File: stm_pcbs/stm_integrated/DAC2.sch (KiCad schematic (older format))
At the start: 21 parts, among them P1 BNC, U1 AD8676, U2 AD5791, U3 AD8675

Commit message: working on Kicad of 3rd Dec
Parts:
- C1, C11, C12, C15, C16, C3, C5, C7, C8: symbol C -> device:C
- C10, C13, C14, C2, C4, C6, C9: symbol CP2 -> device:CP1
- P1: symbol BNC -> device:BNC
- R1: symbol R -> device:R
- U1: symbol AD8676 -> ad5791:AD8676
- U2: symbol AD5791 -> ad5791:AD5791
- U3: symbol AD8675 -> ad5791:AD8675
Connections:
- wire segments 111 -> 126
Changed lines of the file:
@@
-EESchema Schematic File Version 2
-LIBS:power
-LIBS:device
-LIBS:transistors
-LIBS:conn
-LIBS:linear
-LIBS:regul
-LIBS:74xx
-LIBS:cmos4000
-LIBS:adc-dac
-LIBS:memory
-LIBS:xilinx
-LIBS:special
-LIBS:microcontrollers
-LIBS:dsp
-LIBS:microchip
-LIBS:analog_switches
-LIBS:motorola
-LIBS:texas
-LIBS:intel
-LIBS:audio
-LIBS:interface
-LIBS:digital-audio
-LIBS:philips
-LIBS:display
-LIBS:cypress
-LIBS:siliconi
-LIBS:opto
-LIBS:atmel
-LIBS:contrib
-LIBS:valves
-LIBS:ad5791
+EESchema Schematic File Version 4
 LIBS:stmshieldfull-cache
-LIBS:powerbrd-cache
-LIBS:LTC1859-cache
-EELAYER 25 0
+EELAYER 26 0
 EELAYER END
 $Descr A4 11693 8268
@@
 $EndDescr
 $Comp
-L AD5791 U2
+L ad5791:AD5791 U2
 U 1 1 5A25EB42
 P 5050 3750
@@
 $EndComp
 $Comp
-L AD8675 U3
+L ad5791:AD8675 U3
 U 1 1 5A25EB49
 P 6750 3400
@@
 $EndComp
 $Comp
-L AD8676 U1
+L ad5791:AD8676 U1
 U 1 1 5A25EB50
 P 4950 1700
@@
 $EndComp
 $Comp
-L AD8676 U1
+L ad5791:AD8676 U1
 U 2 1 5A25EB57
 P 5000 5450
@@
 $EndComp
 $Comp
-L AD8676 U1
+L ad5791:AD8676 U1
 U 3 1 5A25EB5E
 P 7700 5550
@@
 $EndComp
 $Comp
-L BNC P1
+L device:BNC P1
 U 1 1 5A25EB65
 P 7850 3400
@@
 -14V
 $Comp
-L AGND #PWR01
+L power:AGND #PWR01
 U 1 1 5A25EB72
 P 7850 3750
@@
 3.3V
 $Comp
-L AGND #PWR02
+L power:AGND #PWR02
 U 1 1 5A25EB7B
 P 4850 4850
@@
 $EndComp
 $Comp
-L DGND #PWR03
+L power:DGND #PWR03
 U 1 1 5A25EB81
 P 4600 4850
@@
 $EndComp
 $Comp
-L C C3
+L device:C C3
 U 1 1 5A25EB87
 P 5850 2150
@@
 $EndComp
 $Comp
-L AGND #PWR04
+L power:AGND #PWR04
 U 1 1 5A25EB8E
 P 6300 2300
@@
 $EndComp
 $Comp
-L C C5
+L device:C C5
 U 1 1 5A25EB94
 P 6000 4550
@@
 $EndComp
 $Comp
-L AGND #PWR05
+L power:AGND #PWR05
 U 1 1 5A25EB9B
 P 6400 4700
@@
 $EndComp
 $Comp
-L C C1
+L device:C C1
 U 1 1 5A25EBAF
 P 3850 1850
@@
 $EndComp
 $Comp
-L DGND #PWR06
+L power:DGND #PWR06
 U 1 1 5A25EBB6
 P 3600 1650
@@
 $EndComp
 $Comp
-L C C8
+L device:C C8
 U 1 1 5A25EBBC
 P 7350 5550
@@
 $EndComp
 $Comp
-L C C15
+L device:C C15
 U 1 1 5A25EBC3
 P 8750 5400
@@
 $EndComp
 $Comp
-L C C16
+L device:C C16
 U 1 1 5A25EBCA
 P 8750 5950
@@
 $EndComp
 $Comp
-L AGND #PWR07
+L power:AGND #PWR07
 U 1 1 5A25EBD1
 P 9000 5650
@@
 $EndComp
 $Comp
-L AGND #PWR08
+L power:AGND #PWR08
 U 1 1 5A25EBD7
 P 9000 6200
@@
 $EndComp
 $Comp
-L C C7
+L device:C C7
 U 1 1 5A25EBDD
 P 7100 5550
@@
 $EndComp
 $Comp
-L CP2 C13
+L device:CP1 C13
 U 1 1 5A25EBE4
 P 8500 5400
@@
 $EndComp
 $Comp
-L CP2 C14
+L device:CP1 C14
 U 1 1 5A25EBEB
 P 8500 5950
@@
 $EndComp
 $Comp
-L CP2 C6
+L device:CP1 C6
 U 1 1 5A25EBF2
 P 6000 4800
@@
 $EndComp
 $Comp
-L CP2 C4
+L device:CP1 C4
 U 1 1 5A25EBF9
 P 5850 2400
@@
 $EndComp
 $Comp
-L CP2 C2
+L device:CP1 C2
 U 1 1 5A25EC00
 P 4100 1850
@@
 RESET2
 $Comp
-L CP2 C9
+L device:CP1 C9
 U 1 1 5A25EC0E
 P 7400 3050
@@
 $EndComp
 $Comp
-L CP2 C10
+L device:CP1 C10
 U 1 1 5A25EC15
 P 7400 3800
@@
 $EndComp
 $Comp
-L C C11
+L device:C C11
 U 1 1 5A25EC1C
 P 7600 3050
@@
 $EndComp
 $Comp
-L C C12
+L device:C C12
 U 1 1 5A25EC23
 P 7600 3800
@@
 $EndComp
 $Comp
-L AGND #PWR09
+L power:AGND #PWR09
 U 1 1 5A25EC2A
 P 7300 3250
@@
 $EndComp
 $Comp
-L AGND #PWR010
+L power:AGND #PWR010
 U 1 1 5A25EC30
 P 7400 4100
@@
 	5900 3300 6450 3300
 Wire Wire Line
-	7050 3400 7700 3400
+	7050 3400 7150 3400
 Wire Wire Line
 	4900 1300 4900 1450
@@
 	4900 5700 4900 5850
 Wire Wire Line
-	7250 5200 7800 5200
-Wire Wire Line
-	7250 5900 7800 5900
+	7250 5200 7600 5200
 Wire Wire Line
 	6450 3500 5900 3500
@@
 Connection ~ 7150 3400
 Wire Wire Line
-	6750 3050 6950 3050
-Wire Wire Line
-	6750 3750 6900 3750
+	6750 3050 6850 3050
+Wire Wire Line
+	6750 3750 6850 3750
 Wire Wire Line
 	7850 3600 7850 3750
 Wire Wire Line
-	5600 2000 5600 2300
+	5600 2000 5600 2150
 Wire Wire Line
 	5300 4650 5300 4800
@@
 	4800 2350 4800 2550
 Wire Wire Line
-	4200 2350 4800 2350
+	4200 2350 4450 2350
 Wire Wire Line
 	4650 2350 4650 2550
@@
 Connection ~ 5600 2250
 Wire Wire Line
-	6050 2150 6050 2400
+	6050 2150 6050 2250
 Wire Wire Line
 	6050 2250 6300 2250
@@
 	5300 4650 5800 4650
 Wire Wire Line
-	5800 4550 5800 4800
-Wire Wire Line
-	6200 4550 6200 4800
+	5800 4550 5800 4650
+Wire Wire Line
+	6200 4550 6200 4650
 Connection ~ 5800 4650
 Wire Wire Line
@@
 Connection ~ 6200 4650
 Wire Wire Line
-	3850 1650 4100 1650
-Wire Wire Line
-	3850 2050 4100 2050
-Wire Wire Line
-	3950 2050 4450 2050
+	3850 1650 3950 1650
 Wire Wire Line
 	4450 2050 4450 2350
 Connection ~ 4450 2350
-Connection ~ 3950 2050
 Wire Wire Line
 	3950 1650 3950 1400
@@
 Connection ~ 3950 1650
 Wire Wire Line
-	8500 5200 8750 5200
+	8500 5200 8600 5200
 Wire Wire Line
 	8500 5600 8750 5600
 Wire Wire Line
-	7750 5750 8750 5750
-Wire Wire Line
 	8500 6150 8750 6150
 Wire Wire Line
-	7100 5350 7350 5350
-Wire Wire Line
-	7100 5750 7350 5750
+	7100 5350 7250 5350
+Wire Wire Line
+	7100 5750 7250 5750
 Wire Wire Line
 	7250 5350 7250 5200
@@
 Wire Wire Line
 	7250 5750 7250 5900
-Connection ~ 7600 5900
 Connection ~ 7250 5750
 Wire Wire Line
-	7600 5900 7750 5900
-Wire Wire Line
 	7750 5900 7750 5750
-Connection ~ 8500 5750
 Wire Wire Line
 	7600 5200 7600 5100
@@
 	8750 5650 9000 5650
 Wire Wire Line
-	8750 5550 8750 5650
+	8750 5550 8750 5600
 Wire Wire Line
 	8750 6200 9000 6200
 Wire Wire Line
-	8750 6100 8750 6200
+	8750 6100 8750 6150
 Wire Wire Line
 	3200 4050 3850 4050
@@
 Connection ~ 7700 5900
 Wire Wire Line
-	7400 2850 7600 2850
-Wire Wire Line
-	7300 3250 7600 3250
-Wire Wire Line
-	7400 3600 7600 3600
-Wire Wire Line
 	7400 4000 7600 4000
-Wire Wire Line
-	7500 2850 6850 2850
 Wire Wire Line
 	6850 2850 6850 3050
 Connection ~ 6850 3050
-Connection ~ 7500 2850
-Wire Wire Line
-	7500 3600 6850 3600
 Wire Wire Line
 	6850 3600 6850 3750
 Connection ~ 6850 3750
-Connection ~ 7500 3600
-Connection ~ 7400 4000
-Connection ~ 7400 3250
-$Comp
-L R R1
+$Comp
+L device:R R1
 U 1 1 5A25ECAA
 P 7150 4500
@@
 $EndComp
 $Comp
-L AGND #PWR011
+L power:AGND #PWR011
 U 1 1 5A25ECB1
 P 6900 4600
@@
 $EndComp
 $Comp
-L DGND #PWR012
+L power:DGND #PWR012
 U 1 1 5A25ECB7
 P 7400 4600
@@
 Wire Wire Line
 	8750 5200 8750 5250
+Wire Wire Line
+	7150 3400 7700 3400
+Wire Wire Line
+	4650 2350 4800 2350
+Wire Wire Line
+	5600 2150 5600 2250
+Wire Wire Line
+	5600 2250 5600 2300
+Wire Wire Line
+	6050 2250 6050 2400
+Wire Wire Line
+	5800 4650 5800 4800
+Wire Wire Line
+	6200 4650 6200 4800
+Wire Wire Line
+	4450 2350 4650 2350
+Wire Wire Line
+	3950 1650 4100 1650
+Wire Wire Line
+	7600 5200 7700 5200
+Wire Wire Line
+	7250 5350 7350 5350
+Wire Wire Line
+	7250 5750 7350 5750
+Wire Wire Line
+	8600 5200 8750 5200
+Wire Wire Line
+	7700 5200 7800 5200
+Wire Wire Line
+	6850 3050 6950 3050
+Wire Wire Line
+	6850 3750 6900 3750
+Wire Wire Line
+	8750 6150 8750 6200
+Wire Wire Line
+	8750 5600 8750 5650
+Wire Wire Line
+	7750 5750 8750 5750
+Wire Wire Line
+	7300 3250 7600 3250
+Wire Wire Line
+	3850 2050 4450 2050
+Wire Wire Line
+	7250 5900 7700 5900
+Wire Wire Line
+	7700 5900 7800 5900
+Wire Wire Line
+	6850 2850 7600 2850
+Wire Wire Line
+	6850 3600 7600 3600
 $EndSCHEMATC

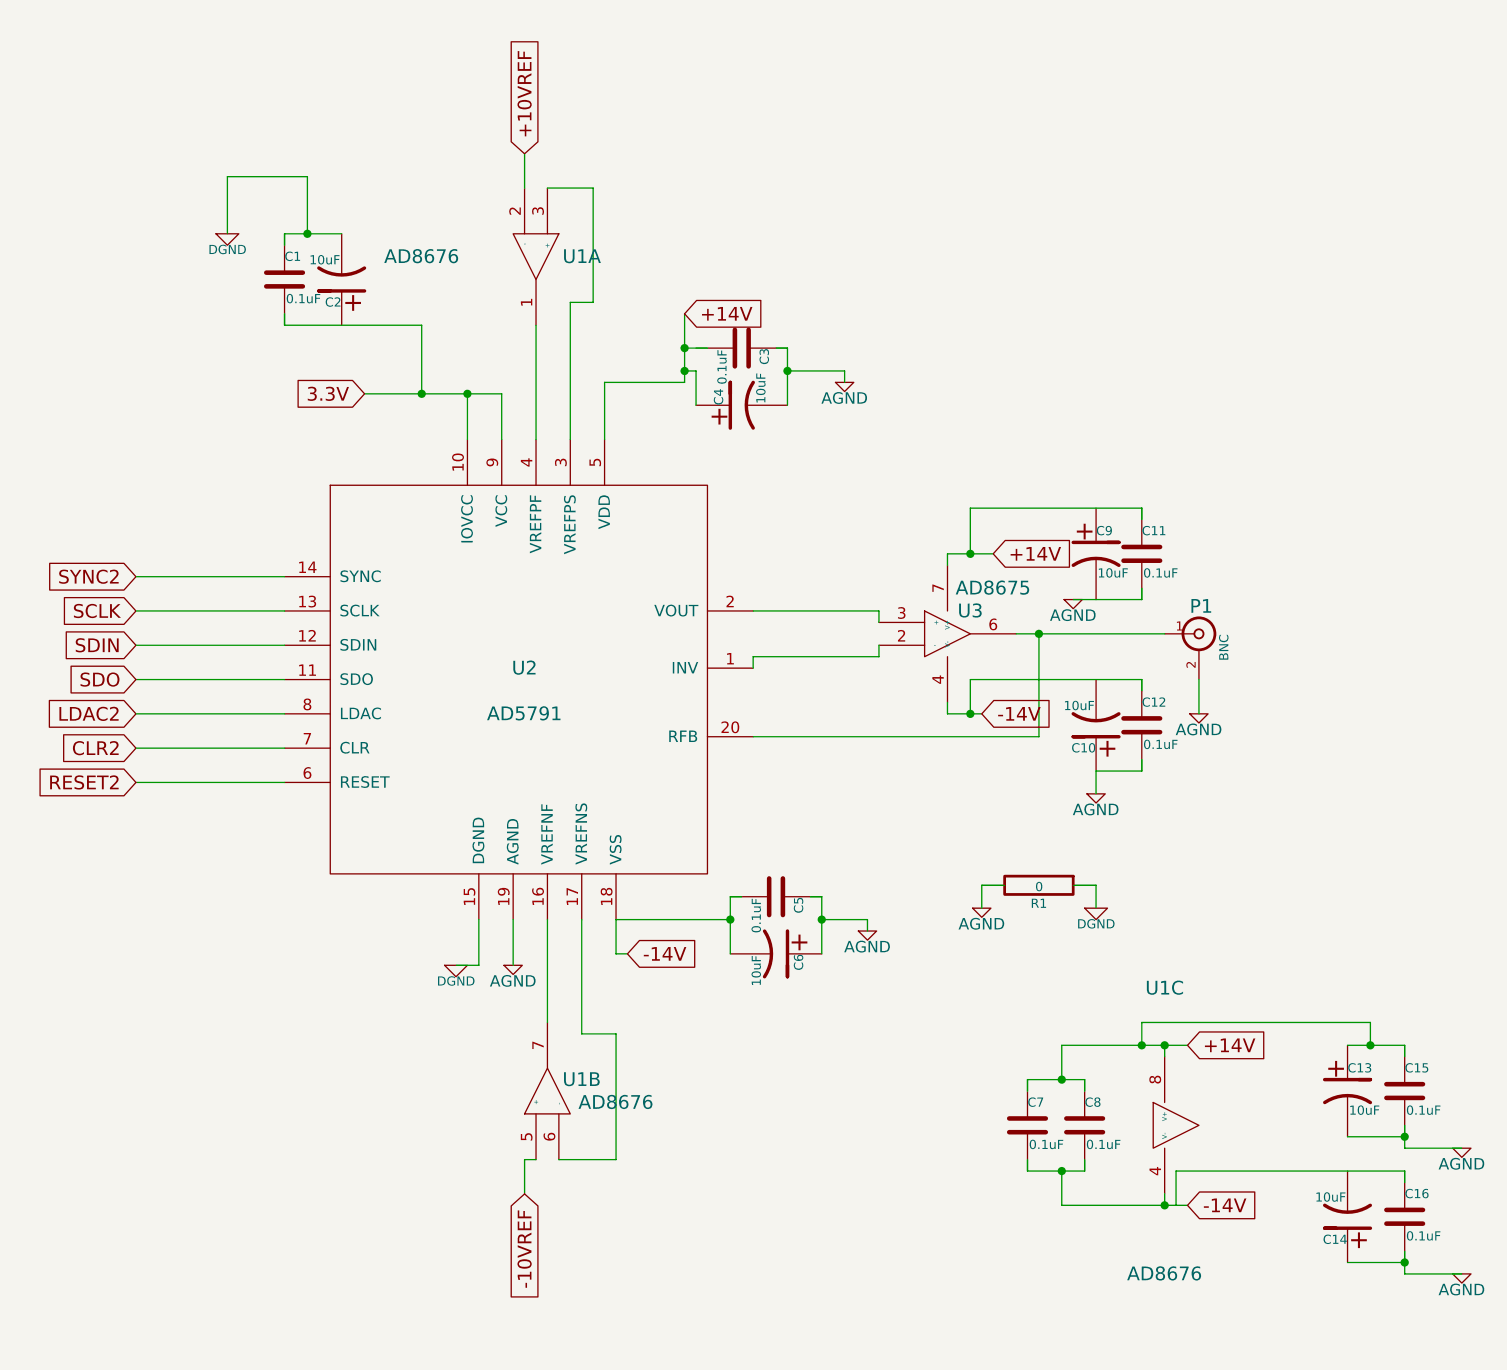
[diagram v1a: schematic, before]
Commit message: fixing more borkage
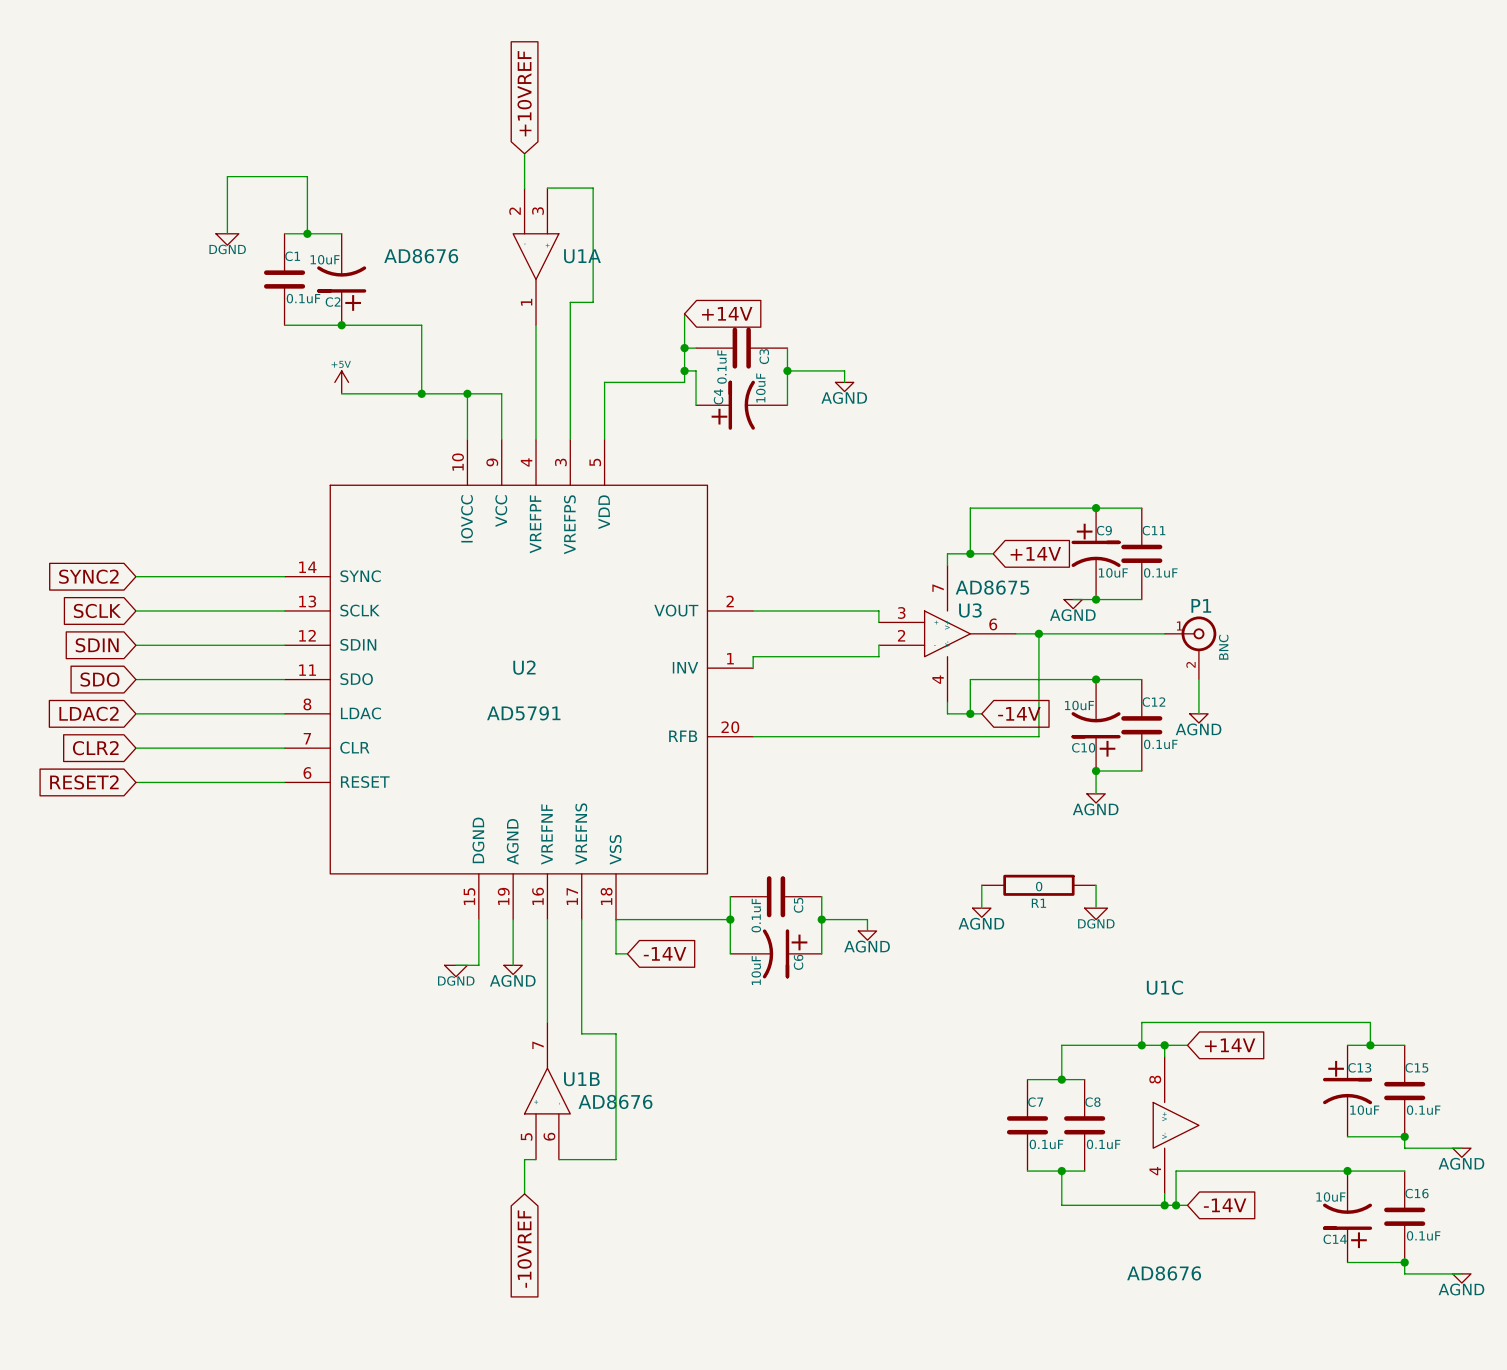
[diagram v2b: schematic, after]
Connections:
- net labels added: +5V
- net labels removed: 3.3V
- wire segments 126 -> 113
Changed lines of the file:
@@
 Text GLabel 5350 4800 2    60   Input ~ 0
 -14V
-Text GLabel 4200 2350 0    60   Input ~ 0
-3.3V
 $Comp
 L power:AGND #PWR02
@@
 	4800 2350 4800 2550
 Wire Wire Line
-	4200 2350 4450 2350
-Wire Wire Line
 	4650 2350 4650 2550
 Connection ~ 4650 2350
@@
 	5250 2300 5250 2550
 Wire Wire Line
-	5600 2150 5700 2150
+	5600 2150 5650 2150
 Connection ~ 5600 2150
 Wire Wire Line
@@
 Connection ~ 7250 5750
 Wire Wire Line
-	7750 5900 7750 5750
-Wire Wire Line
 	7600 5200 7600 5100
 Wire Wire Line
@@
 	8750 5650 9000 5650
 Wire Wire Line
-	8750 5550 8750 5600
-Wire Wire Line
 	8750 6200 9000 6200
-Wire Wire Line
-	8750 6100 8750 6150
 Wire Wire Line
 	3200 4050 3850 4050
@@
 	6900 4500 6900 4600
 Wire Wire Line
-	7600 3600 7600 3650
-Wire Wire Line
-	7600 4000 7600 3950
-Wire Wire Line
-	7400 4500 7300 4500
-Wire Wire Line
-	7000 4500 6900 4500
-Wire Wire Line
-	6150 4550 6200 4550
-Wire Wire Line
-	5850 4550 5800 4550
-Wire Wire Line
-	7600 2850 7600 2900
-Wire Wire Line
-	7600 3250 7600 3200
-Wire Wire Line
-	3850 2000 3850 2050
-Wire Wire Line
-	3850 1700 3850 1650
-Wire Wire Line
-	6000 2150 6050 2150
-Wire Wire Line
 	3200 3150 3850 3150
 Wire Wire Line
 	7400 4100 7400 4000
-Wire Wire Line
-	7350 5350 7350 5400
-Wire Wire Line
-	7350 5750 7350 5700
-Wire Wire Line
-	7100 5750 7100 5700
-Wire Wire Line
-	7100 5400 7100 5350
-Wire Wire Line
-	8750 5750 8750 5800
 Connection ~ 8750 6150
 Connection ~ 8750 5600
 Wire Wire Line
-	8750 5200 8750 5250
-Wire Wire Line
 	7150 3400 7700 3400
 Wire Wire Line
@@
 	8750 5600 8750 5650
 Wire Wire Line
-	7750 5750 8750 5750
-Wire Wire Line
-	7300 3250 7600 3250
-Wire Wire Line
-	3850 2050 4450 2050
+	7750 5750 8500 5750
+Wire Wire Line
+	7300 3250 7400 3250
+Wire Wire Line
+	3850 2050 4100 2050
 Wire Wire Line
 	7250 5900 7700 5900
 Wire Wire Line
-	7700 5900 7800 5900
-Wire Wire Line
-	6850 2850 7600 2850
-Wire Wire Line
-	6850 3600 7600 3600
+	7700 5900 7750 5900
+Wire Wire Line
+	6850 2850 7400 2850
+Wire Wire Line
+	6850 3600 7400 3600
+Connection ~ 7400 3600
+Wire Wire Line
+	7400 3600 7600 3600
+Connection ~ 7400 4000
+Connection ~ 7400 2850
+Wire Wire Line
+	7400 2850 7600 2850
+Connection ~ 7400 3250
+Wire Wire Line
+	7400 3250 7600 3250
+Connection ~ 4100 2050
+Wire Wire Line
+	4100 2050 4450 2050
+Wire Wire Line
+	7750 5750 7750 5900
+Connection ~ 7750 5900
+Wire Wire Line
+	7750 5900 7800 5900
+Connection ~ 8500 5750
+Wire Wire Line
+	8500 5750 8750 5750
+$Comp
+L power:+5V #PWR?
+U 1 1 5A4DE733
+P 4100 2350
+F 0 "#PWR?" H 4100 2440 20  0001 C CNN
+F 1 "+5V" H 4096 2478 30  0000 C CNN
+F 2 "" H 4100 2350 60  0001 C CNN
+F 3 "" H 4100 2350 60  0001 C CNN
+	1    4100 2350
+	1    0    0    -1
+$EndComp
+Wire Wire Line
+	4100 2350 4450 2350
 $EndSCHEMATC
